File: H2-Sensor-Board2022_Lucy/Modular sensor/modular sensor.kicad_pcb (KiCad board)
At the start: 2 copper layers, 41.4 x 20.8 mm, 9 parts, among them J1 Conn_01x03_Pin

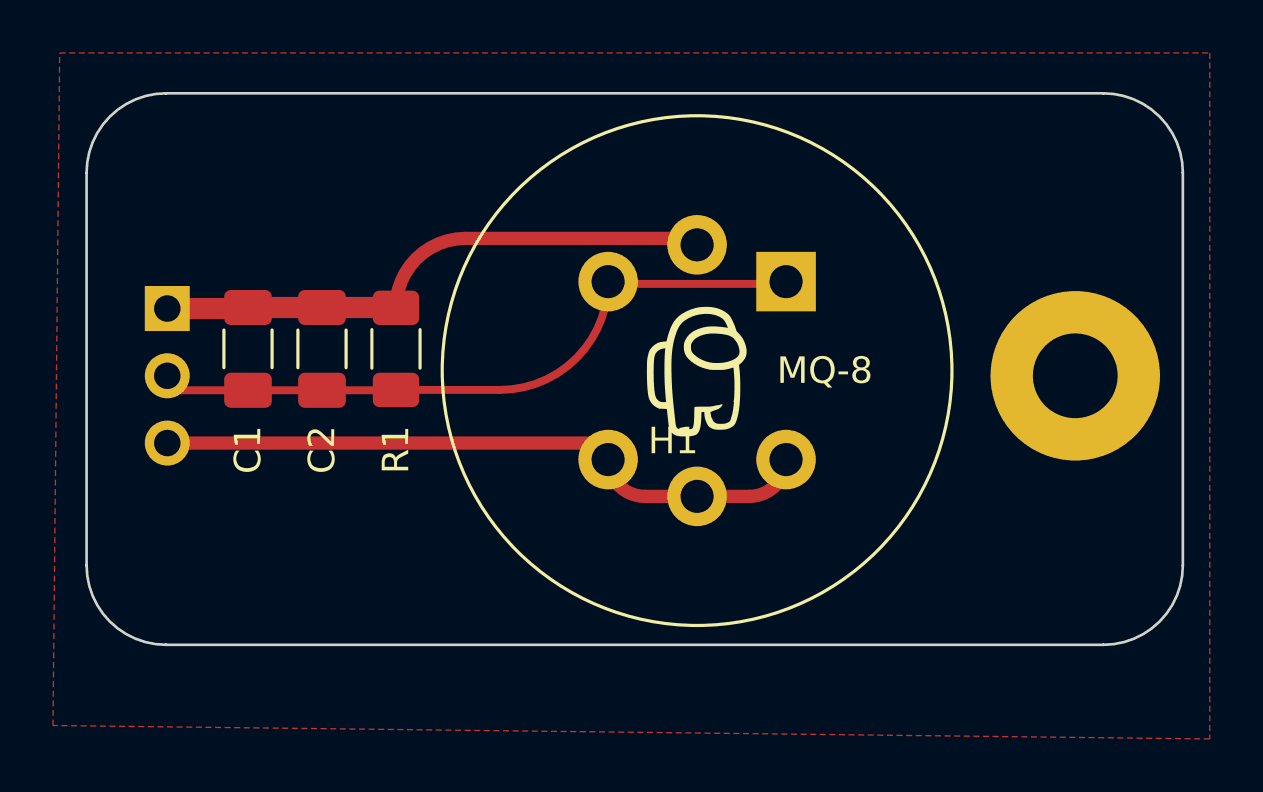
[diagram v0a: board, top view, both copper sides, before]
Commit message: I am highly sleep deprived
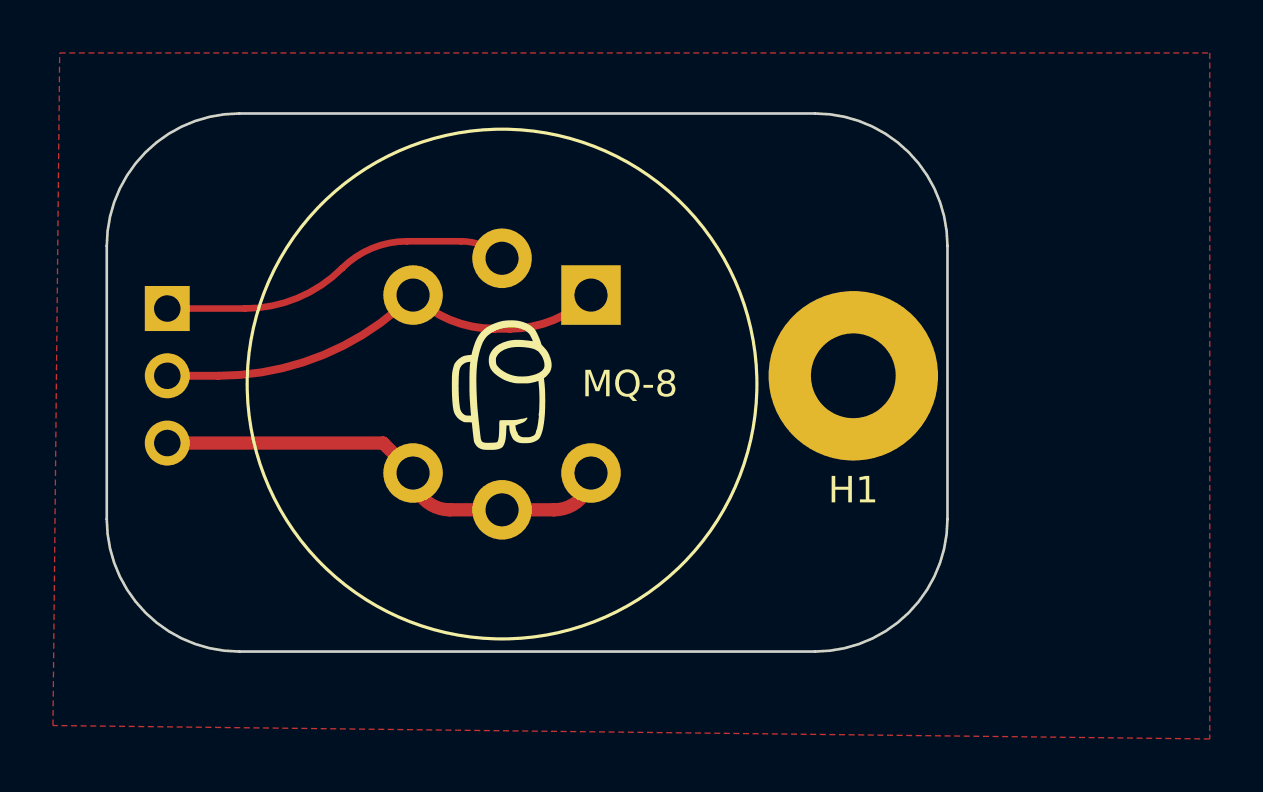
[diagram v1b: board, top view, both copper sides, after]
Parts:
- removed C1: 50nF, Capacitor_SMD:C_1206_3216Metric_Pad1.33x1.80mm_HandSolder
- removed C2: 100uF, Capacitor_SMD:C_1206_3216Metric_Pad1.33x1.80mm_HandSolder
- removed R1: 4k7, Resistor_SMD:R_1206_3216Metric_Pad1.30x1.75mm_HandSolder
- moved G*** 8.61 mm to (144.0, 86.6)
- moved G*** 8.61 mm to (146.5, 86.6)
- moved H1 8.38 mm to (152.9, 94.0)
- moved G*** 7.38 mm to (139.6, 94.3)
- moved MQ-8 7.38 mm to (143.0, 90.9)
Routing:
- net GND: track 21.5 -> 13.4 mm
- net /V_RL: track 25.8 -> 18.3 mm
- net +5V: track 25.1 -> 17.9 mm
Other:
- board size 41.4 x 20.8 mm -> 31.8 x 20.3 mm
- board text removed: "GND"
